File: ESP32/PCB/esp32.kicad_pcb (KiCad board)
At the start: 2 copper layers, 36 x 68.8 mm, 75 parts, among them J1 USB_C_Receptacle_USB2.0_14P, J2 Conn_01x02_Pin, J3 Conn_01x18_Pin, J5 Conn_01x18_Pin, Q1 AO3401A, U1 ESP32-S3, U2 W25Q128JVS, U3 MCP73831-2-OT, U4 AMS1117-3.3, Y1 32.768 kHz, Y2 40MHz(10ppm)

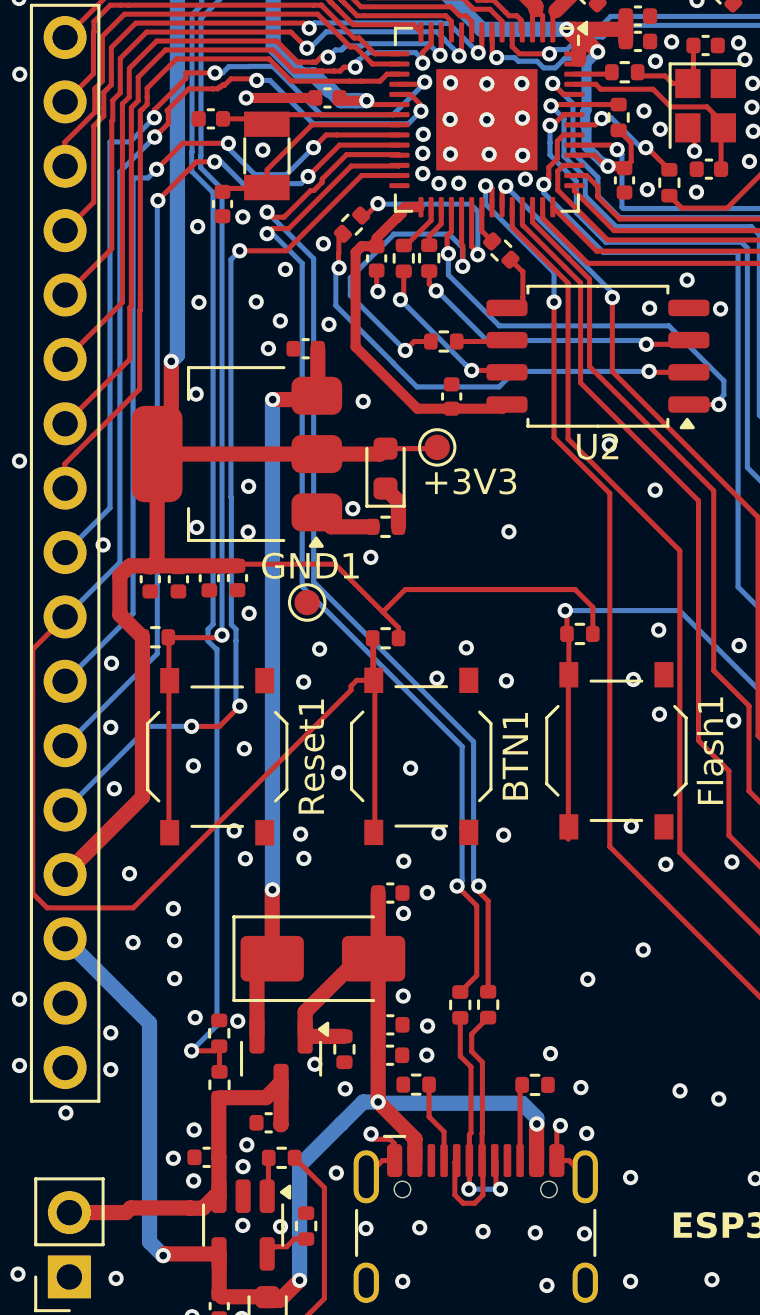
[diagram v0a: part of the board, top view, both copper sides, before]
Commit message: Add files via upload
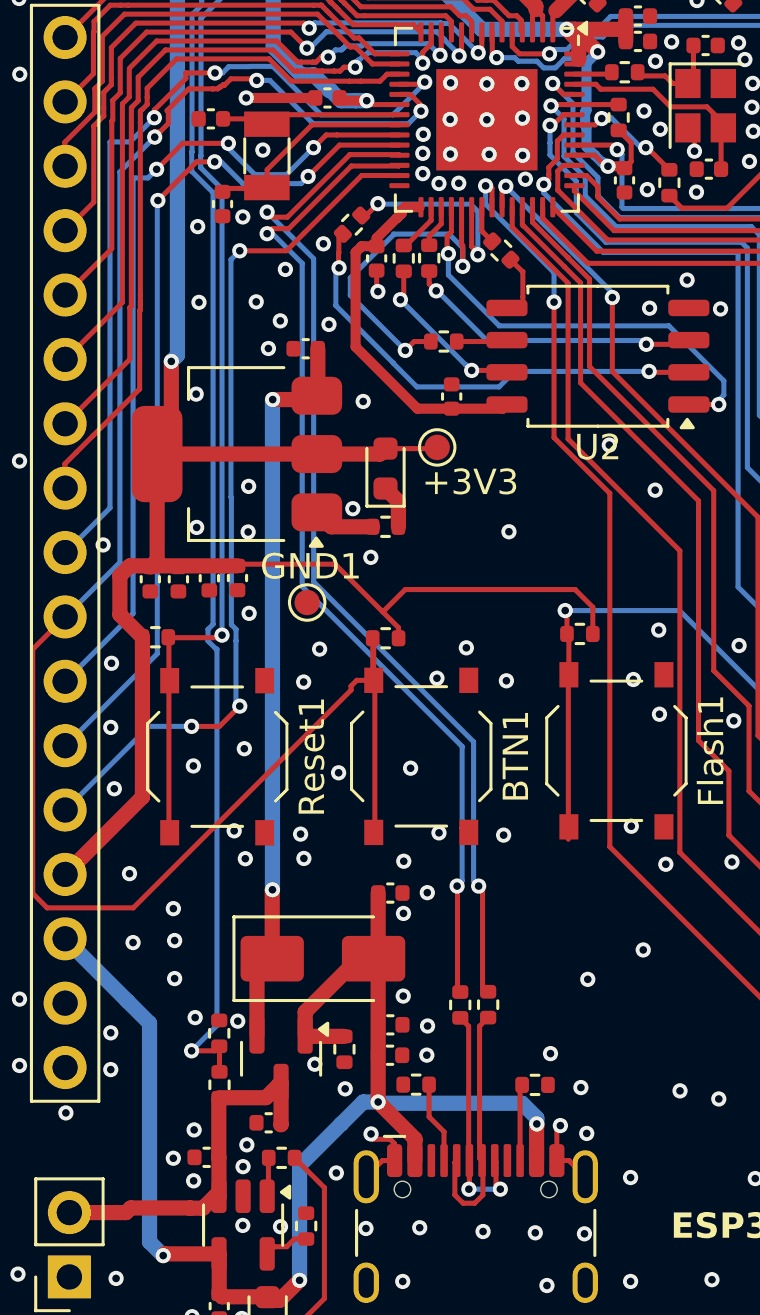
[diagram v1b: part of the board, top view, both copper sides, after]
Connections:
- J1 pad A6: USB_D+ -> Net-(J1-D+-PadA6)
- J1 pad A7: USB_D- -> Net-(J1-D--PadA7)
- J1 pad B6: USB_D+ -> Net-(J1-D+-PadA6)
- J1 pad B7: USB_D- -> Net-(J1-D--PadA7)
- R18 pad 1: USB_D+ -> Net-(J1-D+-PadA6)
- R2 pad 1: USB_D- -> Net-(J1-D--PadA7)
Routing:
- net USB_D-: track 51.2 -> 40.7 mm
- net USB_D+: track 49.7 -> 39.7 mm, vias 4 -> 2
- net Net-(J1-D--PadA7): track 0.00 -> 9.83 mm
- net Net-(J1-D+-PadA6): track 0.00 -> 9.38 mm, vias 0 -> 2
